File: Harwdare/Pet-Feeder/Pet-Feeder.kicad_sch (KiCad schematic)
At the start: 19 parts

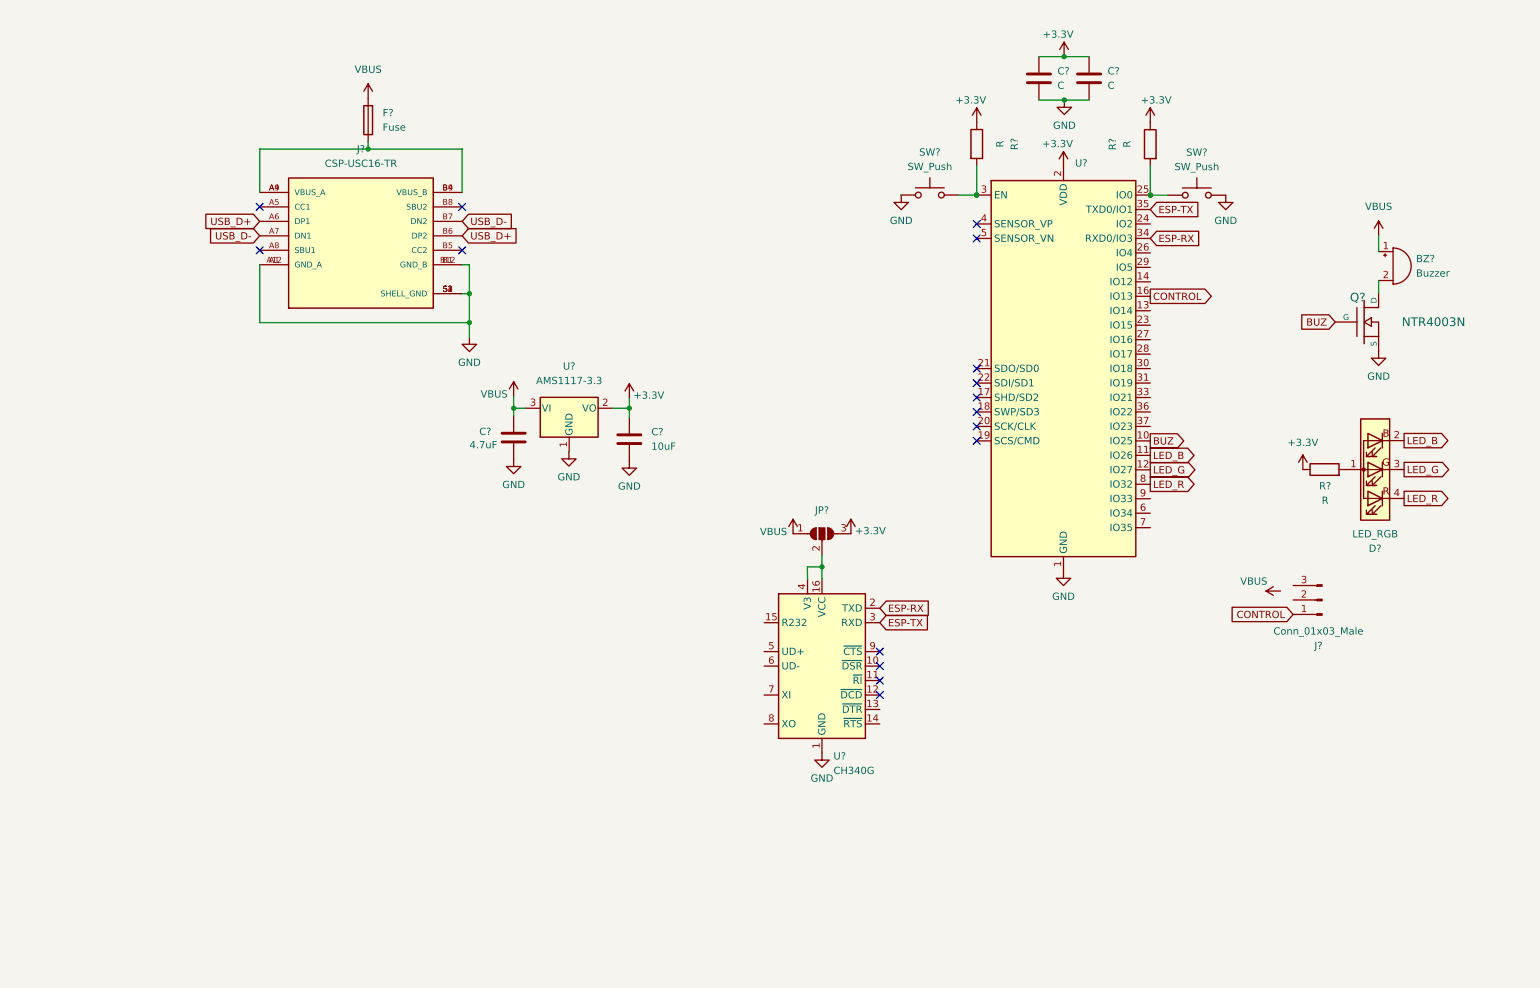
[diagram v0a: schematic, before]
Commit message: Terminei o esquematico
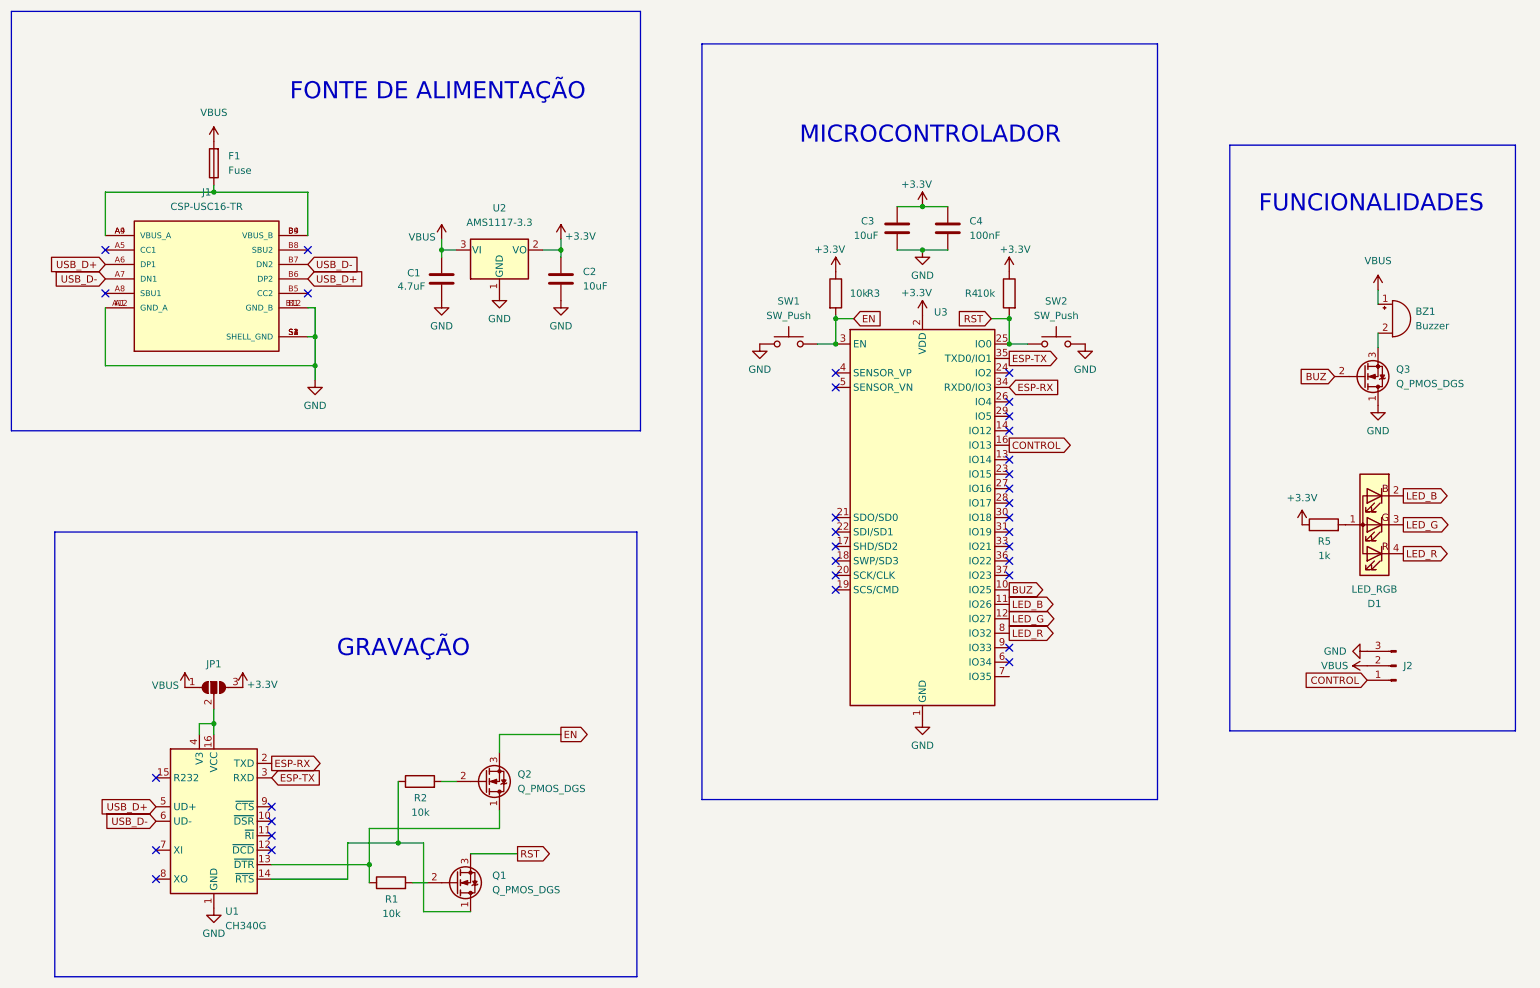
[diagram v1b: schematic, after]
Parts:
- removed Q?: NTR4003N, SOT23GDS, symbol esp32-rescue:MOSFET_N
- added Q1, Q2, Q3: Q_PMOS_DGS, Package_TO_SOT_SMD:SOT-23-3, symbol Device:Q_NMOS_DGS
- added R1, R2: 10k, Resistor_SMD:R_0201_0603Metric, symbol Device:R
- C3: renamed from C?; value C -> 10uF
- C4: renamed from C?; value C -> 100nF
- J2: renamed from J?; footprint (none) -> Connector_PinSocket_2.54mm:PinSocket_1x03_P2.54mm_Vertical
- JP1: renamed from JP?; footprint (none) -> Jumper:SolderJumper-3_P1.3mm_Open_RoundedPad1.0x1.5mm
- R3, R4: renamed from R?; value R -> 10k
- R5: renamed from R?; value R -> 1k
- SW1, SW2: renamed from SW?; footprint (none) -> Button_Switch_SMD:SW_Push_1P1T_NO_CK_KSC6xxJ
- gave numbers to parts that had none: 9
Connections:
- net BUZ: now also Q3.2 (G)
- net GND: now also J2.3 (Pin_3), Q3.1 (D)
- net USB_D+: now also U1.5 (UD+)
- net USB_D-: now also U1.6 (UD-)
- net VBUS: now also J2.2 (Pin_2)
- net EN: now reaches R3.2, U3.3 (EN)
- net EN: now also SW1.2, Q2.3 (S)
- net RST: now reaches SW2.2
- net RST: now also R4.2, U3.25 (IO0), Q1.3 (S)
- net at U1.13 (~{DTR}): now also Q2.1 (D), R1.1
- net at U1.14 (~{RTS}): now also Q1.1 (D), R2.1
- net at BZ1.2 (+): now also Q3.3 (S)
- new net: Q1.2 (G), R1.2
- new net: Q2.2 (G), R2.2
- no-connect marks 16 -> 34
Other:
- note added: "FONTE DE ALIMENTAÇÃO"
- note added: "FUNCIONALIDADES"
- note added: "GRAVAÇÃO"
- note added: "MICROCONTROLADOR"
- moved on the sheet: BZ1, C1, C2, C3, C4, D1, F1, J1, J2, JP1, R3, R4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
